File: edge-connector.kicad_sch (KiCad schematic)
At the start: 1 part, among them J1 PCB-Edge_DC-SCM-2.1_2x84_Rev-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

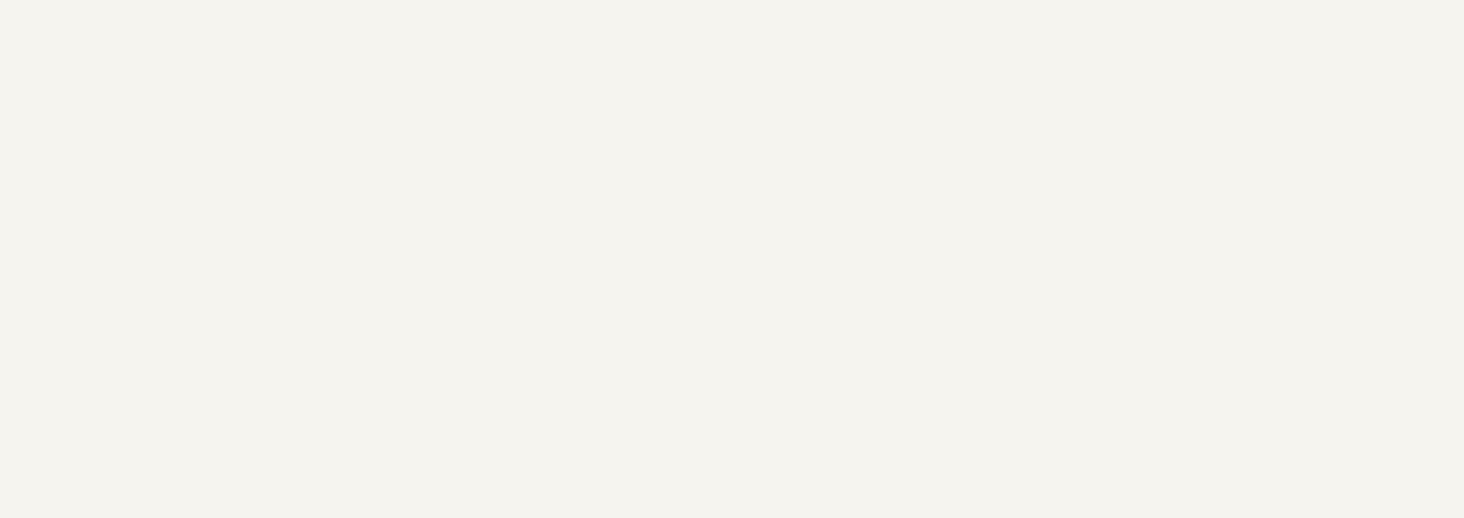
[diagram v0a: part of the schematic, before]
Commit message: [#100720] Add DCDC
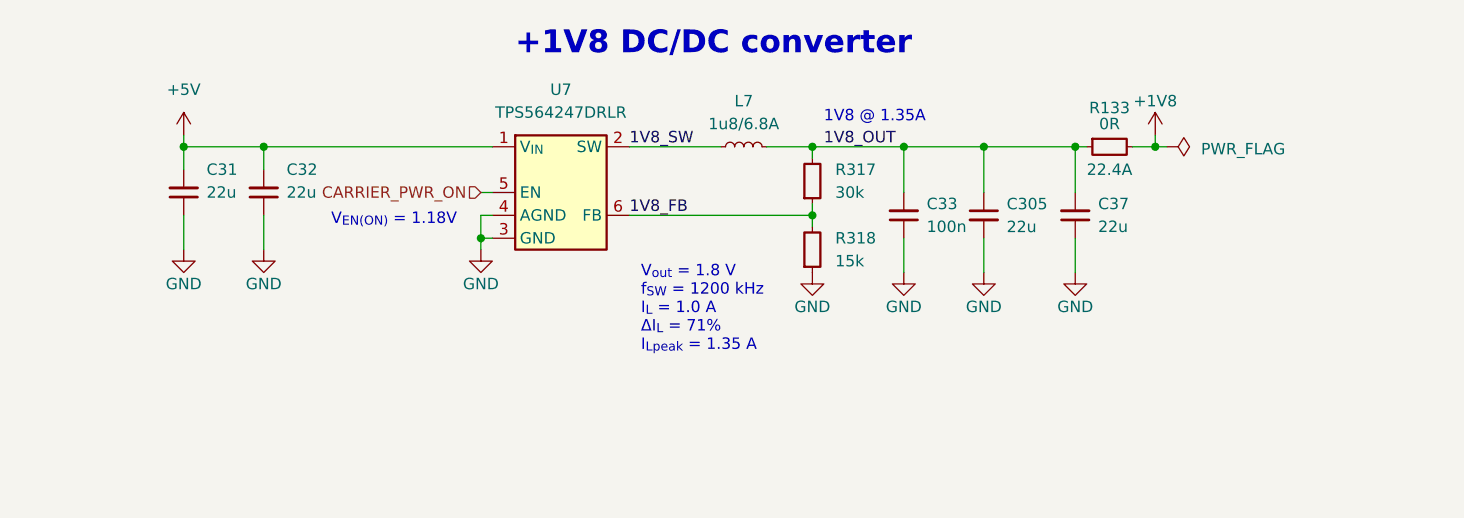
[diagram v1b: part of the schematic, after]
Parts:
- added C305, C31, C32, C37: C_22u_16V_0603, antmicro-footprints:C_0603_1608Metric_EIA, symbol antmicroCapacitors0603:C_22u_16V_0603
- added C33: C_100n_0402, antmicro-footprints:C_0402_1005Metric, symbol antmicroCapacitors0402:C_100n_0402
- added L7: L_1u8_6.8A_WE-MAPI-4020, antmicro-footprints:L_WE-MAPI-4020, symbol antmicroFixedInductors:L_1u8_6.8A_WE-MAPI-4020
- added R133: R_0R_22.4A_0603, antmicro-footprints:R_0603_1608Metric, symbol antmicroResistors0603:R_0R_22.4A_0603
- added R317: R_30k_0402, antmicro-footprints:R_0402_1005Metric, symbol antmicroResistors0402:R_30k_0402
- added R318: R_15k_0402, antmicro-footprints:R_0402_1005Metric, symbol antmicroResistors0402:R_15k_0402
- added U7: TPS564247DRLR, antmicro-footprints:SOT-563, symbol antmicroDCDCConverters:TPS564247DRLR
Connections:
- net GND: now also C305.2, C31.1, C32.1, C33.1, C37.1, R318.1, U7.3 (GND), U7.4 (AGND)
- new net +1V8: R133.2
- new net +5V: C31.2, C32.2, U7.1 (V_{IN})
- new net 1V8_FB: R317.1, R318.2, U7.6 (FB)
- new net 1V8_OUT: C305.1, C33.2, C37.2, L7.2, R133.1, R317.2
- new net 1V8_SW: L7.1, U7.2 (SW)
- new net CARRIER_PWR_ON: U7.5 (EN)
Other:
- note added: "+1V8 DC/DC converter"
- note added: "1V8 @ 1.35A"
- note added: "V_{EN(ON)} = 1.18V"
- note added: "V_{out} = 1.8 V f_{SW} = 1200 kHz I_{L} = 1.0 A ΔI_{L} = 71% I_{Lpeak} = 1.35 A"
